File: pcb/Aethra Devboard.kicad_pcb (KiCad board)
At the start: 2 copper layers, 21 x 51 mm, 45 parts, among them J1 USB_C_Receptacle_USB2.0_14P, J2 Conn_01x20, J3 Conn_01x20, J4 Conn_01x03, J5 Conn_01x02, Q1 DMG2301L, SW1 SW_Push, U1 RP2040, U2 AP2112K-3.3, U3 W25Q16JVZPIQ, U4 MCP73831-2-OT, Y1 12 MHz

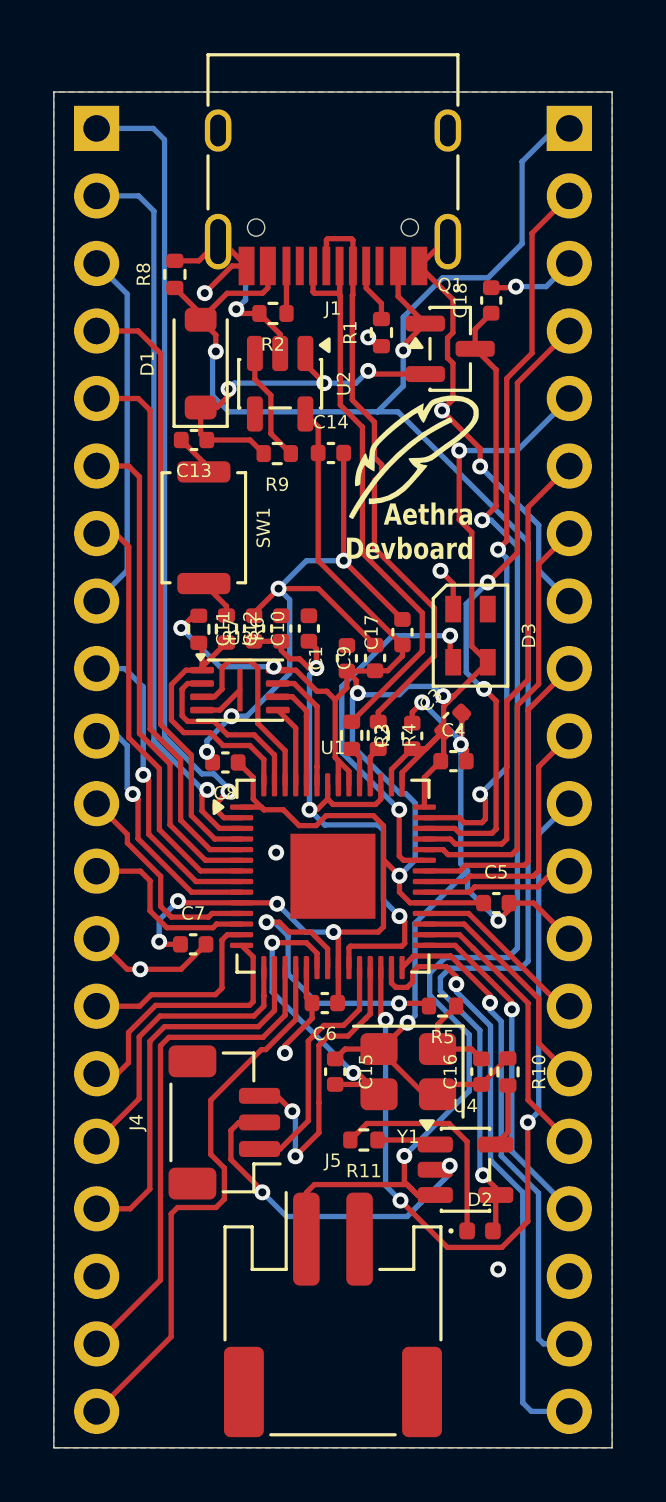
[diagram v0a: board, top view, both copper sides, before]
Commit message: Reroute PCB
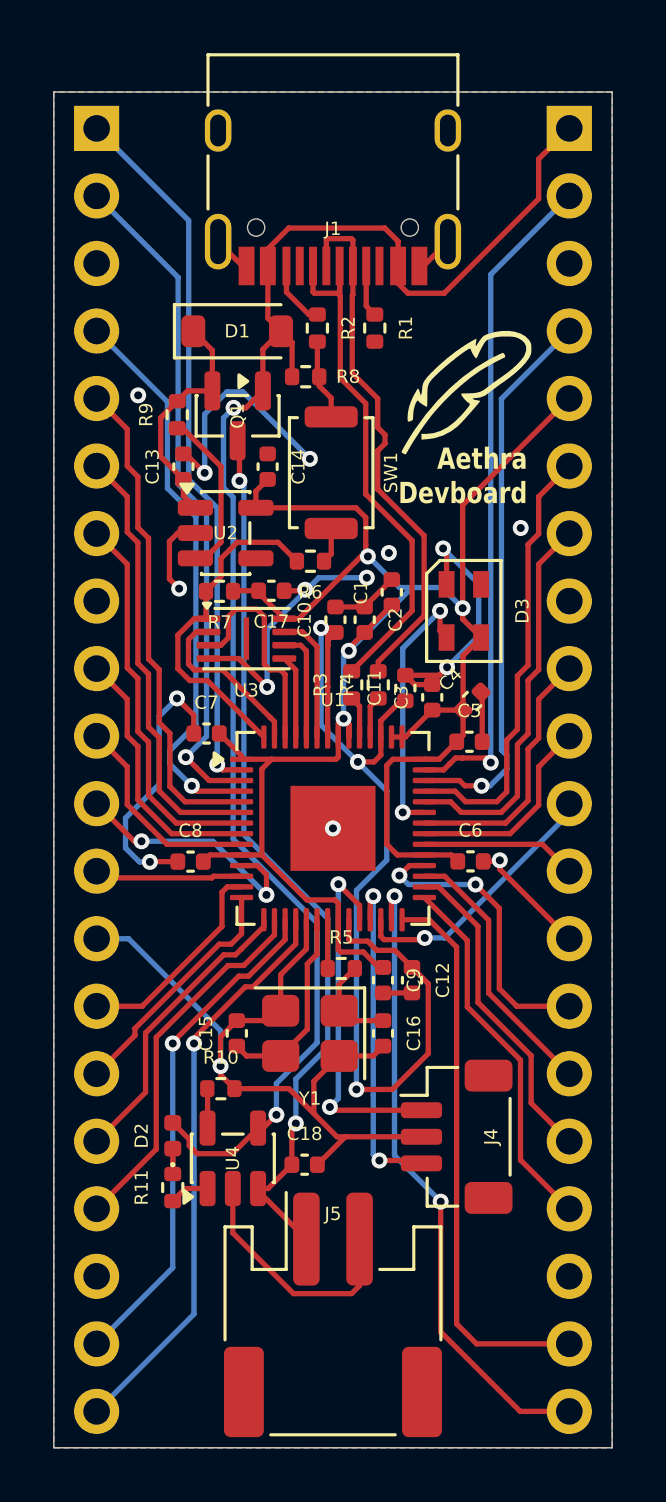
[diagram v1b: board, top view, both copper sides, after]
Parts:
- moved C18 33.3 mm to (149.6, 118.5), turned to 0 degrees
- moved C12 14.1 mm to (153.6, 111.5), turned to -90 degrees
- moved C9 12.1 mm to (152.5, 111.5), turned to -90 degrees
- moved D2 12.1 mm to (144.6, 117.4), turned to 90 degrees
- moved R10 10.8 mm to (146.4, 115.6), turned to 180 degrees
- moved U4 8.76 mm to (146.9, 118.2), turned to 90 degrees
- moved J4 8.76 mm to (155.3, 117.4), turned to -90 degrees
- moved Q1 8.39 mm to (147.0, 90.3), turned to -90 degrees
- moved C7 7.95 mm to (145.9, 102.2), turned to 180 degrees
- moved C6 7.64 mm to (155.8, 107.0), turned to 0 degrees
- moved R11 7.41 mm to (144.6, 119.3), turned to 90 degrees
- moved R8 6.25 mm to (149.6, 88.8), turned to 0 degrees
- moved C5 6.15 mm to (155.8, 102.5)
- moved C11 6.11 mm to (153.3, 100.5)
- moved U2 5.98 mm to (146.6, 94.7), turned to 0 degrees
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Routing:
- net GND: track 127.6 -> 97.0 mm, vias 21 -> 16
- net RUN: track 31.4 -> 10.1 mm, vias 3 -> 1
- net +3V3: track 95.6 -> 74.9 mm, vias 10 -> 4
- net +1V1: track 24.2 -> 37.6 mm
- net +BATT: track 46.2 -> 33.5 mm
- net VBUS: track 71.4 -> 60.1 mm, vias 3 -> 2
- net XOUT: track 11.7 -> 1.83 mm, vias 2 -> 0
- net Net-(D2-K): track 8.29 -> 0.95 mm
- net Net-(D1-K): track 14.3 -> 8.83 mm, vias 3 -> 0
- net SWCLK: track 9.27 -> 13.7 mm, vias 0 -> 2
- net GPIO21: track 6.90 -> 11.3 mm, vias 0 -> 2
- net XIN: track 11.7 -> 7.49 mm, vias 2 -> 0
- net NEOPIXEL: track 14.2 -> 10.1 mm
- net GPIO0: track 30.5 -> 26.8 mm
- net QSPI_SS: track 10.3 -> 12.9 mm
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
